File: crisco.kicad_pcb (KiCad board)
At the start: 2 copper layers, 213.4 x 38.1 mm, 45 parts, among them J1 LED, J2 OLED, SW1 SW_Push, U1 ProMicro

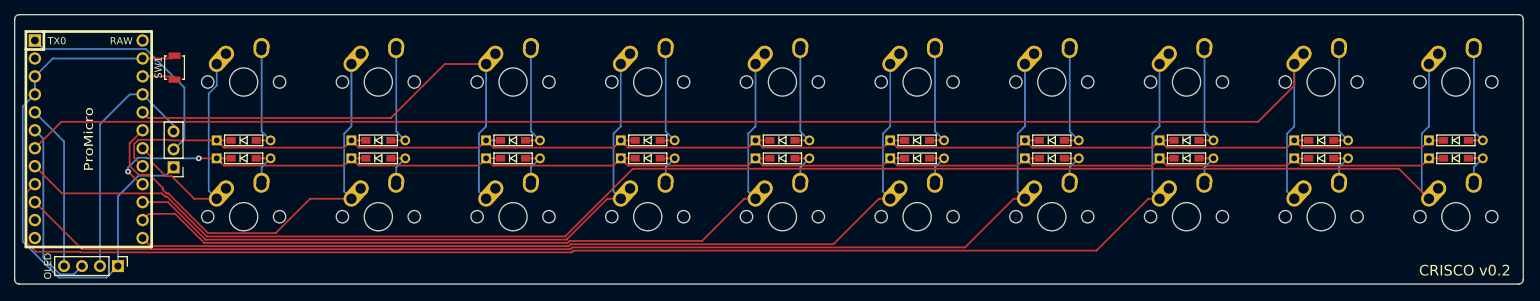
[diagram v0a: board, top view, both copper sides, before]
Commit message: choc hybrid
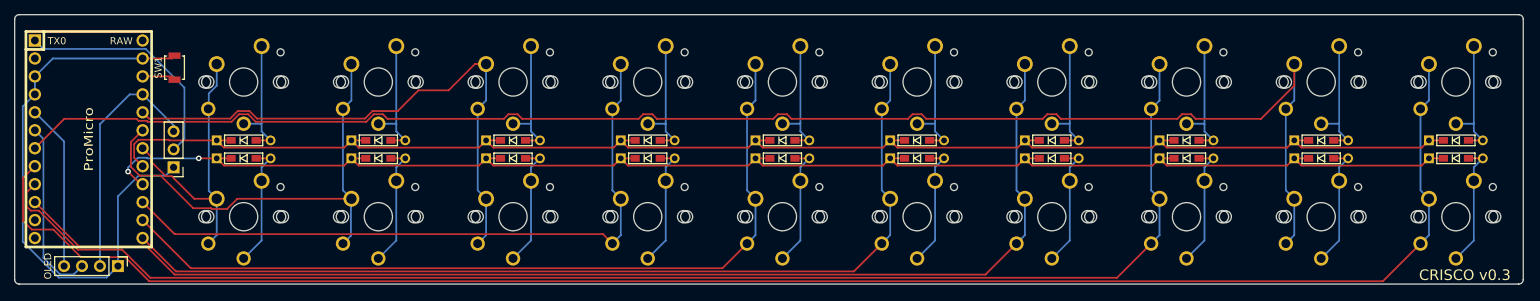
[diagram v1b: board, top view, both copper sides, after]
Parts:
- MX1, MX10, MX11, MX12, MX13, MX14, MX15, MX16, MX17, MX18, MX19, MX2, MX20, MX3, MX4, MX5, MX6, MX7, MX8, MX9: footprint MX_Alps_Hybrid:MX-1U-NoLED -> MX_Alps_Hybrid:MX-Choc-1U-NoLED
- moved G*** 2.87 mm to (211.3, 103.6)
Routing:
- net Net-(D19-Pad2): track 5.74 -> 17.8 mm
- net Net-(D12-Pad2): track 5.74 -> 17.8 mm
- net Net-(D11-Pad2): track 5.74 -> 17.8 mm
- net Net-(D13-Pad2): track 5.74 -> 17.8 mm
- net Net-(D16-Pad2): track 5.74 -> 17.8 mm
- net Net-(D20-Pad2): track 5.74 -> 17.8 mm
- net Net-(D18-Pad2): track 5.74 -> 17.8 mm
- net Net-(D17-Pad2): track 5.74 -> 17.8 mm
- net Net-(D15-Pad2): track 5.74 -> 17.8 mm
- net Net-(D14-Pad2): track 5.74 -> 17.8 mm
- net col8: track 204.7 -> 216.7 mm
- net col9: track 226.9 -> 238.7 mm
- net col2: track 72.0 -> 80.0 mm
- net col0: track 34.0 -> 40.8 mm
- net col6: track 165.6 -> 171.8 mm
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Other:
- board text added: "CRISCO v0.3"
- board text removed: "CRISCO v0.2"
